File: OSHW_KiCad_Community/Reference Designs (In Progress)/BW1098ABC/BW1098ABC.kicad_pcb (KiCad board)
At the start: 4 copper layers, 150 x 65.2 mm, 116 parts, among them J1 Conn_02x05_Odd_Even, J13 DF23C-50DP-0.5V_92_, J2 FAN, J3 BW1099EMB_SoM, J4 Conn_02x05_Odd_Even, J5 USBC 3.1 Vertical, J6 26_pin_FFC, J7 26_pin_FFC, J9 26_pin_FFC, Q1 RK7002B, Q2 RK7002B, Q3 RK7002B, Q4 RK7002B, Q5 RK7002B, U1 2-bit bidirectional level shi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, U6 USB Type-C Switch, U7 USB Type-C Port Control

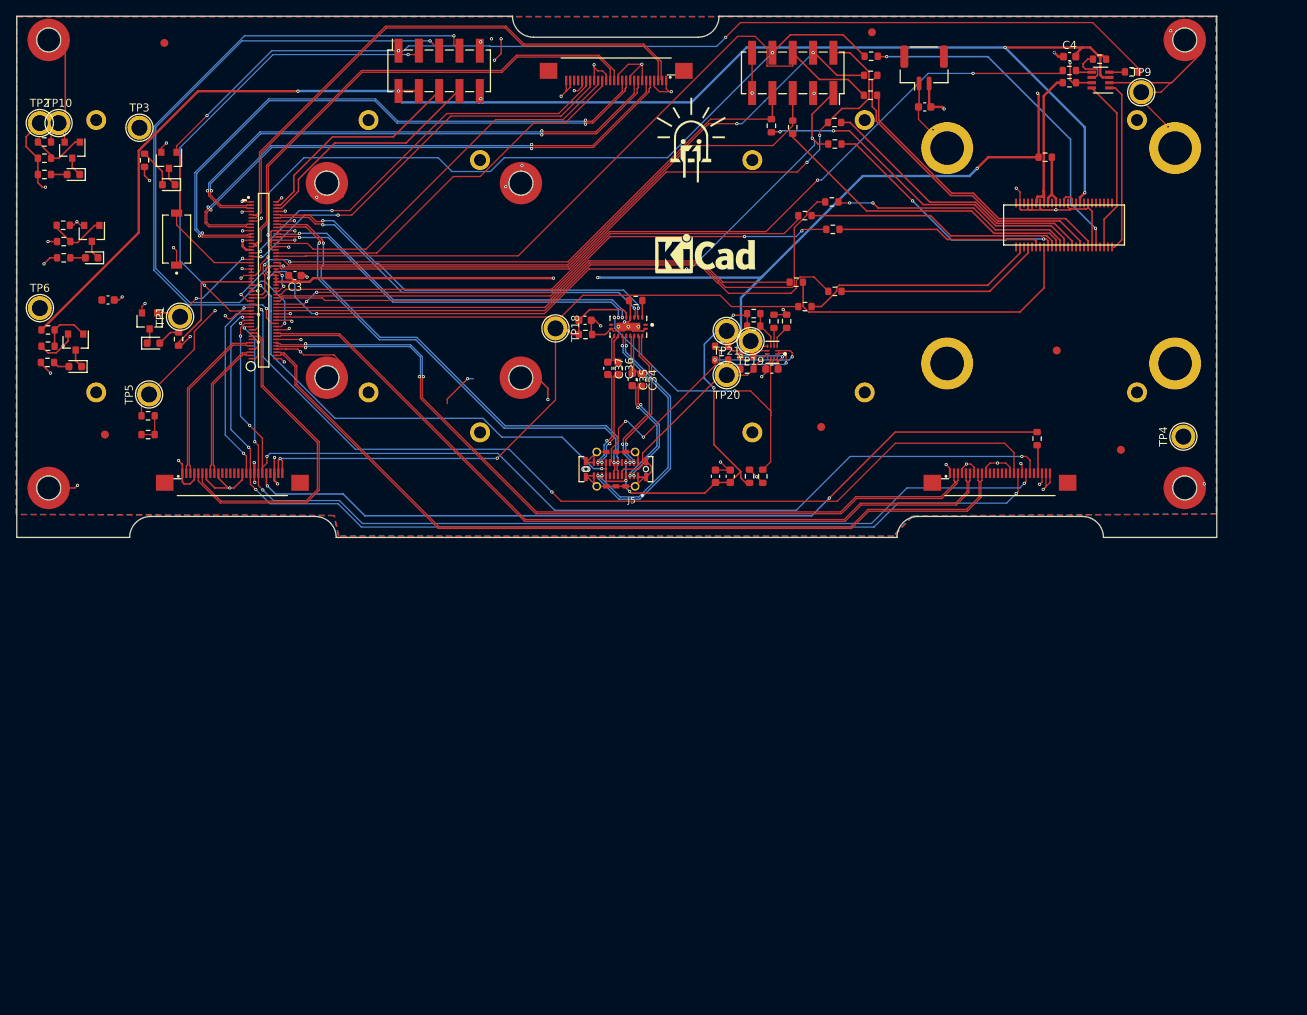
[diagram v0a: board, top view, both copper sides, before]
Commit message: abc updates
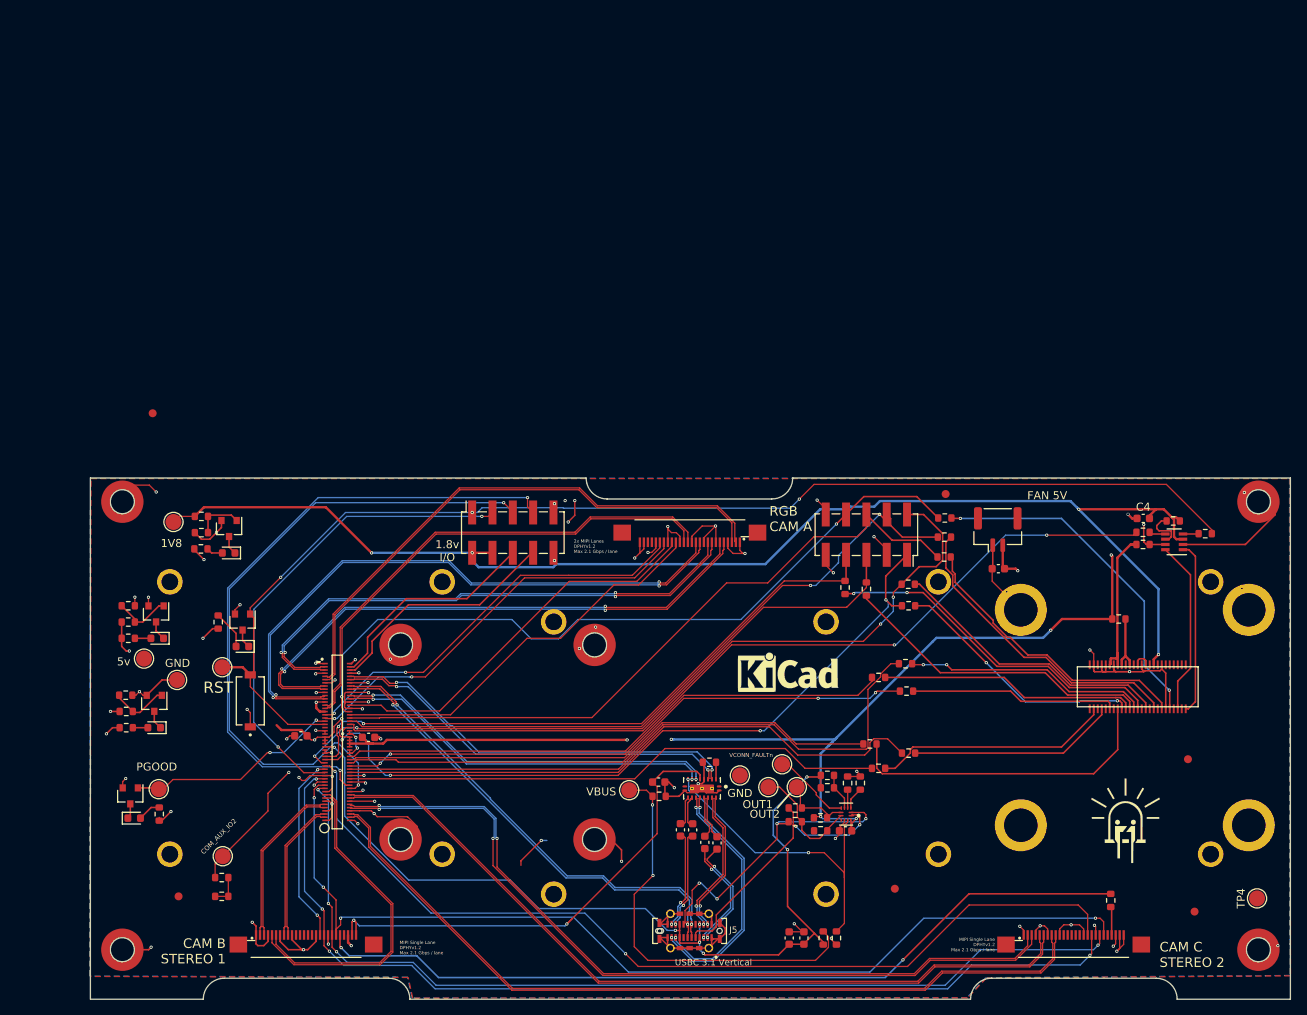
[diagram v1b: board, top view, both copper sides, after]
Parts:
- added REF**: FabDrawing-4Layer, FabDrawingTemplates:FabDrawing-4Layer-Metric_noNotes, F.Cu at (154.2, 18.7)
- TP1, TP10, TP18, TP19, TP2, TP20, TP21, TP3, TP4, TP5, TP6, TP9: footprint TestPoint:TestPoint_Plated_Hole_D2.0mm -> TestPoint:TestPoint_Pad_D2.0mm
- moved G*** 100.9 mm to (257.2, 135.6)
- moved TP9 99.1 mm to (209.0, 130.0)
- moved TP10 71.2 mm to (138.7, 118.0)
- moved TP3 68.2 mm to (144.3, 116.5)
- moved TP2 68.2 mm to (134.6, 115.4)
- moved C1 59.6 mm to (154.2, 125.0), turned to 180 degrees
- moved D2 59.4 mm to (133.3, 135.3)
- moved Q2 59.4 mm to (132.8, 132.5)
- moved R3 59.4 mm to (136.5, 134.8)
- moved D4 59.3 mm to (135.8, 124.0)
- moved Q4 59.3 mm to (135.8, 121.0)
- moved R29 59.3 mm to (132.3, 122.0)
- moved R33 59.3 mm to (132.3, 120.0)
- moved R30 59.3 mm to (132.3, 124.0)
- moved TP1 59.1 mm to (136.4, 131.7)
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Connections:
- R16 pad 2: +3V3 -> Net-(R16-Pad2)
- R32 pad 1: +3V3 -> Net-(R16-Pad2)
- TP18 pad 1: +3V3 -> Net-(R16-Pad2)
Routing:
- net Net-(R16-Pad2): track 0.00 -> 51.0 mm, vias 0 -> 2
- net 1V8: track 187.7 -> 166.6 mm
- net Earth: track 272.0 -> 256.7 mm
- net +5V: track 180.0 -> 165.1 mm
- net /SoM_BW1099/2485_PGOOD: track 15.2 -> 27.4 mm
- net Net-(TP19-Pad1): track 2.40 -> 9.83 mm
- net /USBC&POWER/OUT2: track 8.26 -> 14.6 mm
- net SD_HST0_D2: track 91.6 -> 87.2 mm
- net _RST: track 151.0 -> 154.9 mm
- net USB_D_P: track 61.9 -> 59.0 mm
- net USB_D_N: track 61.4 -> 58.6 mm
- net /USBC&POWER/CC2: track 34.6 -> 36.9 mm
- net +3V3: track 94.3 -> 92.1 mm, vias 11 -> 10
- net SD_HST0_D1: track 86.1 -> 88.2 mm
- net /USBC&POWER/CC1: track 33.2 -> 34.1 mm
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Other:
- board text added: "1.8v I/O"
- board text added: "1V8"
- board text added: "2x MIPI Lanes DPHYv1.2 Max 2.1 Gbps / lane"
- board text added: "5v"
- board text added: "CAM B STEREO 1"
- board text added: "CAM C STEREO 2"
- board text added: "COM_AUX_IO2"
- board text added: "FAN 5V"
- board text added: "GND"
- board text added: "MIPI Single Lane DPHYv1.2 Max 2.1 Gbps / lane"
- board text added: "OUT1"
- board text added: "OUT2"
- board text added: "PGOOD"
- board text added: "RGB CAM A"
- board text added: "RST"
- board text added: "VBUS"
- board text added: "VCONN_FAULTn"
- board text removed: "10. REMOVE ALL BURRS AND BREAK SHARP EDGES R0.003 MIN. 11. NON-DESTRUCTIVE EVALUATION: A. ALL PWBS SHALL PASS 100% ELECTRICAL TEST USING SUPPLIED IPC-356 NETLIST IN ACCORDANCE WITH CURRENT REVISION OF IPC-9252, CLASS 2. B. CERTIFICATE OF CONFORMANCE SHALL BE SUPPLIED WITH EACH SHIPMENT. 12. X-OUTS: A. X-OUT BOARDS THAT DO NOT MEET ALL SPECIFICATIONS USING PERMANENT MARKING ON BOTH SIDES OF THE AF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"
